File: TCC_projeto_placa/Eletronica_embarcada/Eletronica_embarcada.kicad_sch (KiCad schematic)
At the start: 85 parts, among them J3 BOOT_JUMPER, J4 BUZZER

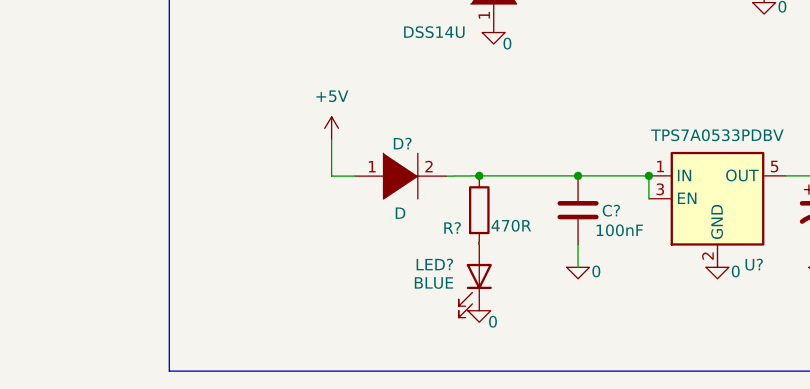
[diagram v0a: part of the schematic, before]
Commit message: aat
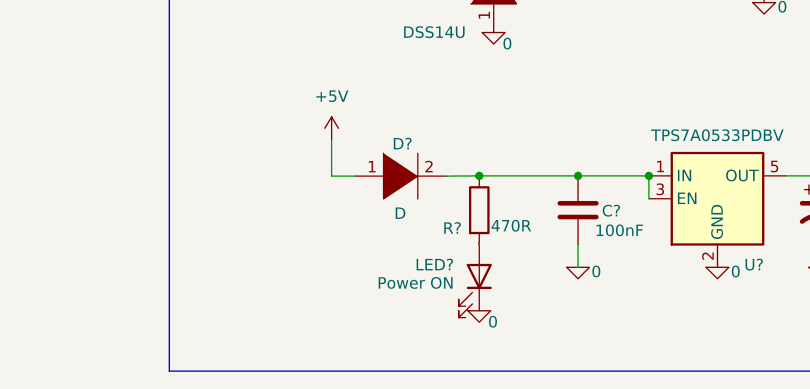
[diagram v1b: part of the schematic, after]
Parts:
- LED?: value BLUE -> Power ON
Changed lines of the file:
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@@
       (effects (font (size 1.27 1.27)) (justify right))
     )
-    (property "Value" "BLUE" (id 1) (at 196.2912 265.5316 90)
+    (property "Value" "Power ON" (id 1) (at 196.2912 265.5316 90)
       (effects (font (size 1.27 1.27)) (justify right))
     )
@@
     )
     (path "/3eb2af48-db14-40c5-89b2-80d6417d5ec9"
-      (reference "LED?") (unit 1) (value "BLUE") (footprint "LED_SMD:LED_0603_1608Metric_Pad1.05x0.95mm_HandSolder")
+      (reference "LED?") (unit 1) (value "Power ON") (footprint "LED_SMD:LED_0603_1608Metric_Pad1.05x0.95mm_HandSolder")
     )
     (path "/0e72554a-372c-4459-91eb-e0cbd9668bdb"
